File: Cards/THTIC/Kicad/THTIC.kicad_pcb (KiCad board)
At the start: 2 copper layers, 55.9 x 33.8 mm, 38 parts, among them J1 Conn_01x04_Pin, J2 Plasma 300V, J3 Plasma 300V, U1 B0509S-1WR3, U2 ISO1540, U3 MCP3221, U4 MCP3221, U5 LMV321, U6 AMS1117-5, U7 LMV321

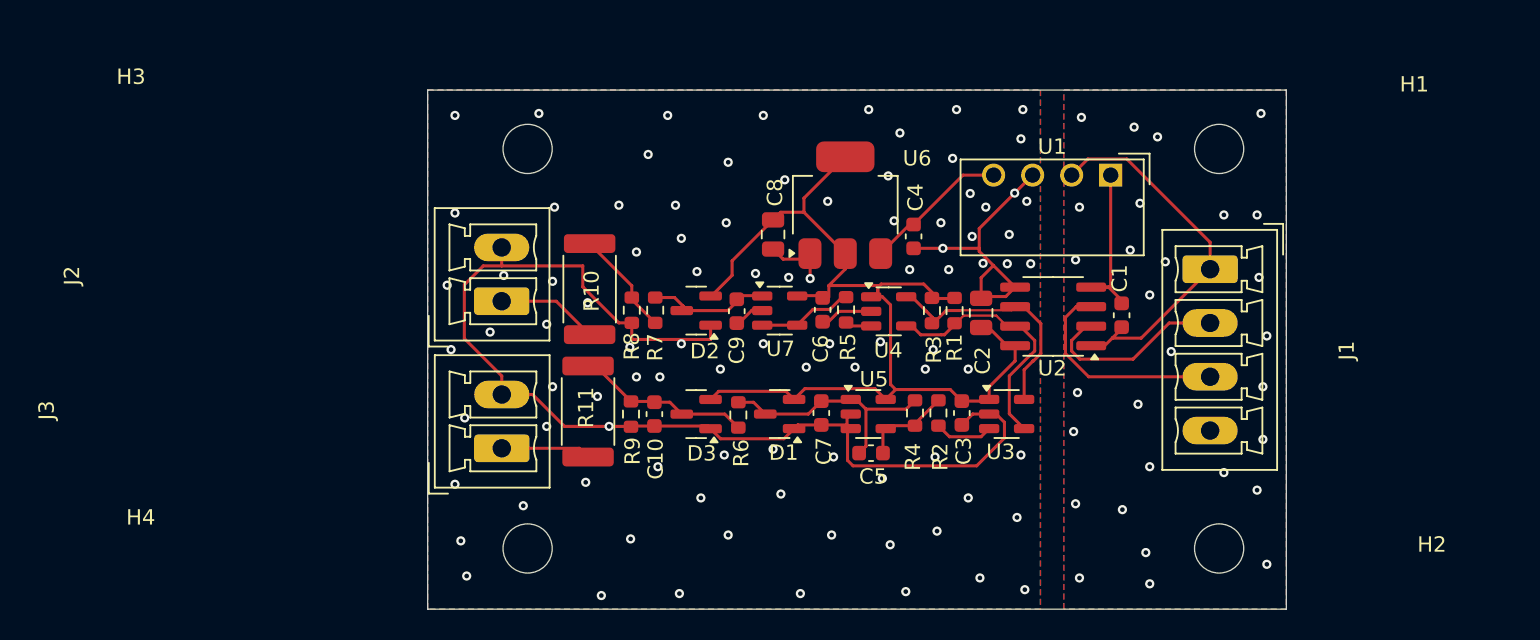
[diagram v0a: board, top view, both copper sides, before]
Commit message: Ordered the real version
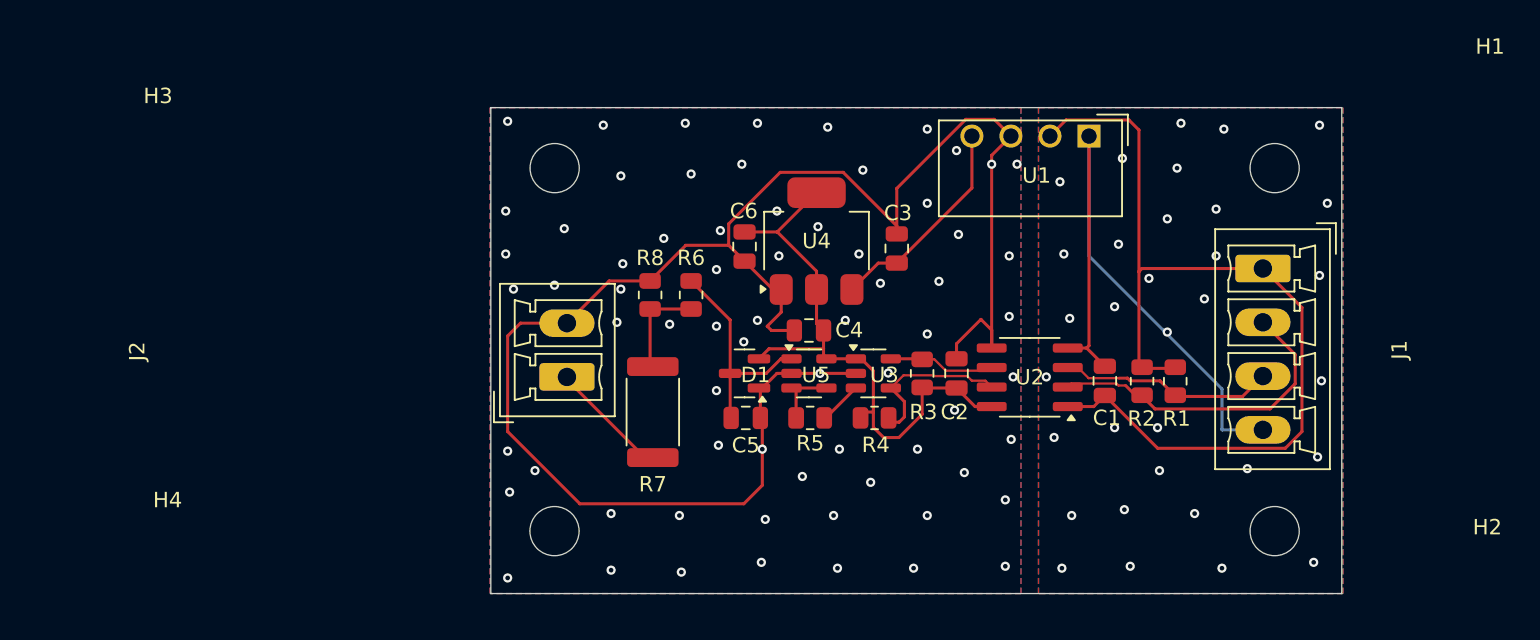
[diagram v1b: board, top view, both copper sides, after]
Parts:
- removed C10: 1nF, Capacitor_SMD:C_0603_1608Metric
- removed the C3 at (177.3, 103.2)
- removed the C5 at (171.3, 105.8)
- removed C7: nP, Capacitor_SMD:C_0603_1608Metric
- removed the D1 at (165.4, 103.3)
- removed D3: BAT54S, Package_TO_SOT_SMD:SOT-23
- removed J3: Plasma 300V, Connector_Phoenix_MC:PhoenixContact_MCV_1,5_2-G-3.5_1x02_P3.50mm_Vertical
- removed R11: 100k, Resistor_SMD:R_2512_6332Metric
- removed the R6 at (162.7, 103.3)
- removed R9: 1k27, Resistor_SMD:R_0603_1608Metric
- removed the U3 at (180.2, 103.3)
- removed the U5 at (171.2, 103.3)
- C1: footprint Capacitor_SMD:C_0603_1608Metric -> Capacitor_SMD:C_0805_2012Metric
- C3: renamed from C4; footprint Capacitor_SMD:C_0603_1608Metric -> Capacitor_SMD:C_0805_2012Metric
- C4: renamed from C6; footprint Capacitor_SMD:C_0603_1608Metric -> Capacitor_SMD:C_0805_2012Metric
- C5: renamed from C9; footprint Capacitor_SMD:C_0603_1608Metric -> Capacitor_SMD:C_0805_2012Metric
- R1: renamed from R4; value 10k -> 2k2; footprint Resistor_SMD:R_0603_1608Metric -> Resistor_SMD:R_0805_2012Metric
- R2: value 47 -> 2k2; footprint Resistor_SMD:R_0603_1608Metric -> Resistor_SMD:R_0805_2012Metric
- R3, R5: footprint Resistor_SMD:R_0603_1608Metric -> Resistor_SMD:R_0805_2012Metric
- R4: renamed from R1; footprint Resistor_SMD:R_0603_1608Metric -> Resistor_SMD:R_0805_2012Metric
- R6: renamed from R7; footprint Resistor_SMD:R_0603_1608Metric -> Resistor_SMD:R_0805_2012Metric
- R8: value 1k27 -> 2k7; footprint Resistor_SMD:R_0603_1608Metric -> Resistor_SMD:R_0805_2012Metric
- moved R1 17.1 mm to (191.1, 101.1), turned to -90 degrees
- moved R2 13.4 mm to (189.0, 101.1), turned to -90 degrees
- moved R7 9.00 mm to (157.1, 103.1)
- moved R4 8.71 mm to (171.6, 103.5), turned to 0 degrees
- moved R5 7.41 mm to (167.4, 103.5), turned to 180 degrees
- moved C5 6.97 mm to (163.2, 103.5), turned to 0 degrees
- moved J2 6.51 mm to (151.6, 100.8)
- moved D1 5.16 mm to (163.1, 100.6)
- moved U5 4.51 mm to (167.3, 100.6)
- moved C1 4.40 mm to (186.6, 101.1)
- moved C2 4.25 mm to (176.9, 100.6)
- moved U2 4.24 mm to (181.7, 100.9)
- moved U3 4.16 mm to (171.5, 100.6)
- moved R3 4.14 mm to (174.7, 100.6), turned to 90 degrees
- moved H1 3.82 mm to (197.6, 87.2)
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- renumbered C8 to C6, D2 to D1, R10 to R7, U4 to U3, U6 to U4, U7 to U5
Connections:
- R1 pad 1: Net-(C5-Pad2) -> 5V
- R1 pad 2: Net-(D1-COM) -> Net-(J1-Pin_3)
- R2 pad 1: Net-(U3-AIN) -> 5V
- R2 pad 2: Net-(C5-Pad2) -> Net-(J1-Pin_2)
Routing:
- net 5V: track 23.4 -> 61.5 mm
- net GND: track 11.1 -> 42.1 mm, vias 29 -> 33
- net VCC_ISO: track 65.8 -> 38.2 mm
- net Net-(D1-COM): track 15.2 -> 0.00 mm
- net GND_ISO: track 100.1 -> 111.8 mm, vias 92 -> 69
- net Net-(D3-COM): track 10.9 -> 0.00 mm
- net Net-(J1-Pin_2): track 12.2 -> 21.1 mm
- net Net-(U2-SCL2): track 15.0 -> 6.63 mm
- net Net-(D2-COM): track 8.23 -> 14.6 mm
- net Net-(J3-Pin_1): track 5.85 -> 0.00 mm
- net Net-(U2-SDA2): track 15.8 -> 10.5 mm
- net Net-(C5-Pad2): track 5.28 -> 0.00 mm
- net Net-(U1-+Vout): track 9.22 -> 13.9 mm
- net Net-(U3-AIN): track 3.82 -> 0.00 mm
- net Net-(U7--): track 5.96 -> 3.96 mm
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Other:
- board size 55.9 x 33.8 mm -> 55.4 x 31.6 mm
- board text added: "MetalMusings THTIC"
- board text removed: "MetalMusings THCIC prototype 1"
